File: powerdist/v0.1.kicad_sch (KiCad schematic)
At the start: 29 parts, among them J1 Conn_01x02_Socket, J2 Conn_01x02_Socket, J3 Conn_01x02_Socket, J4 Conn_01x02_Socket

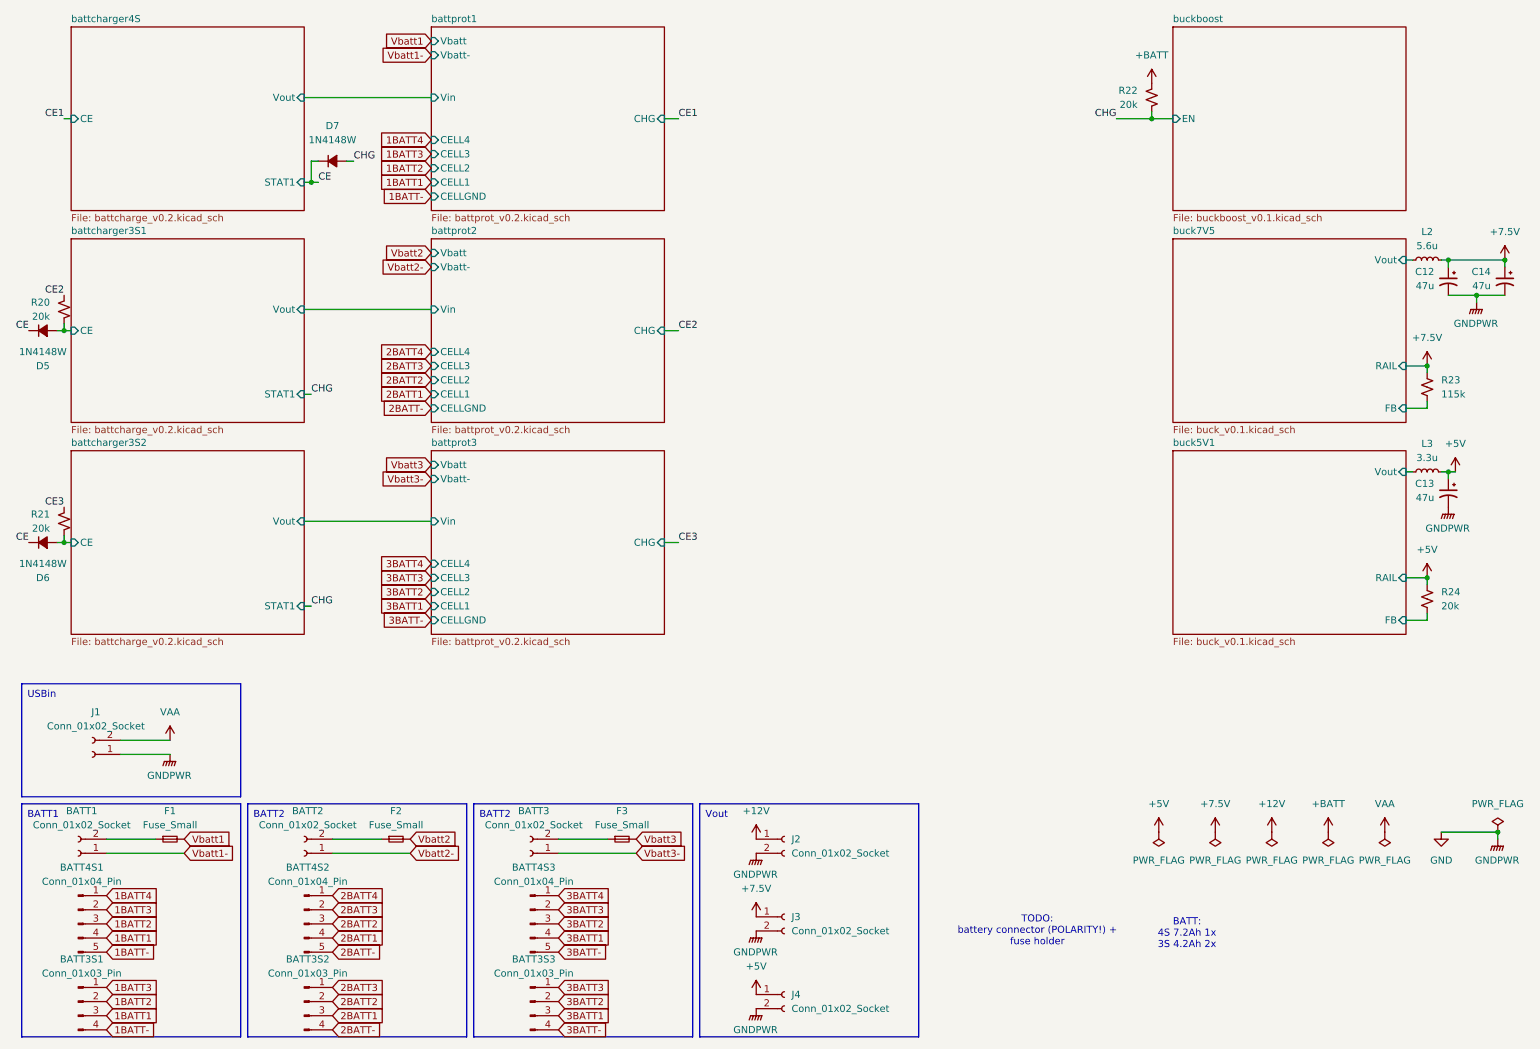
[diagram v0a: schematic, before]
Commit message: local 19/10
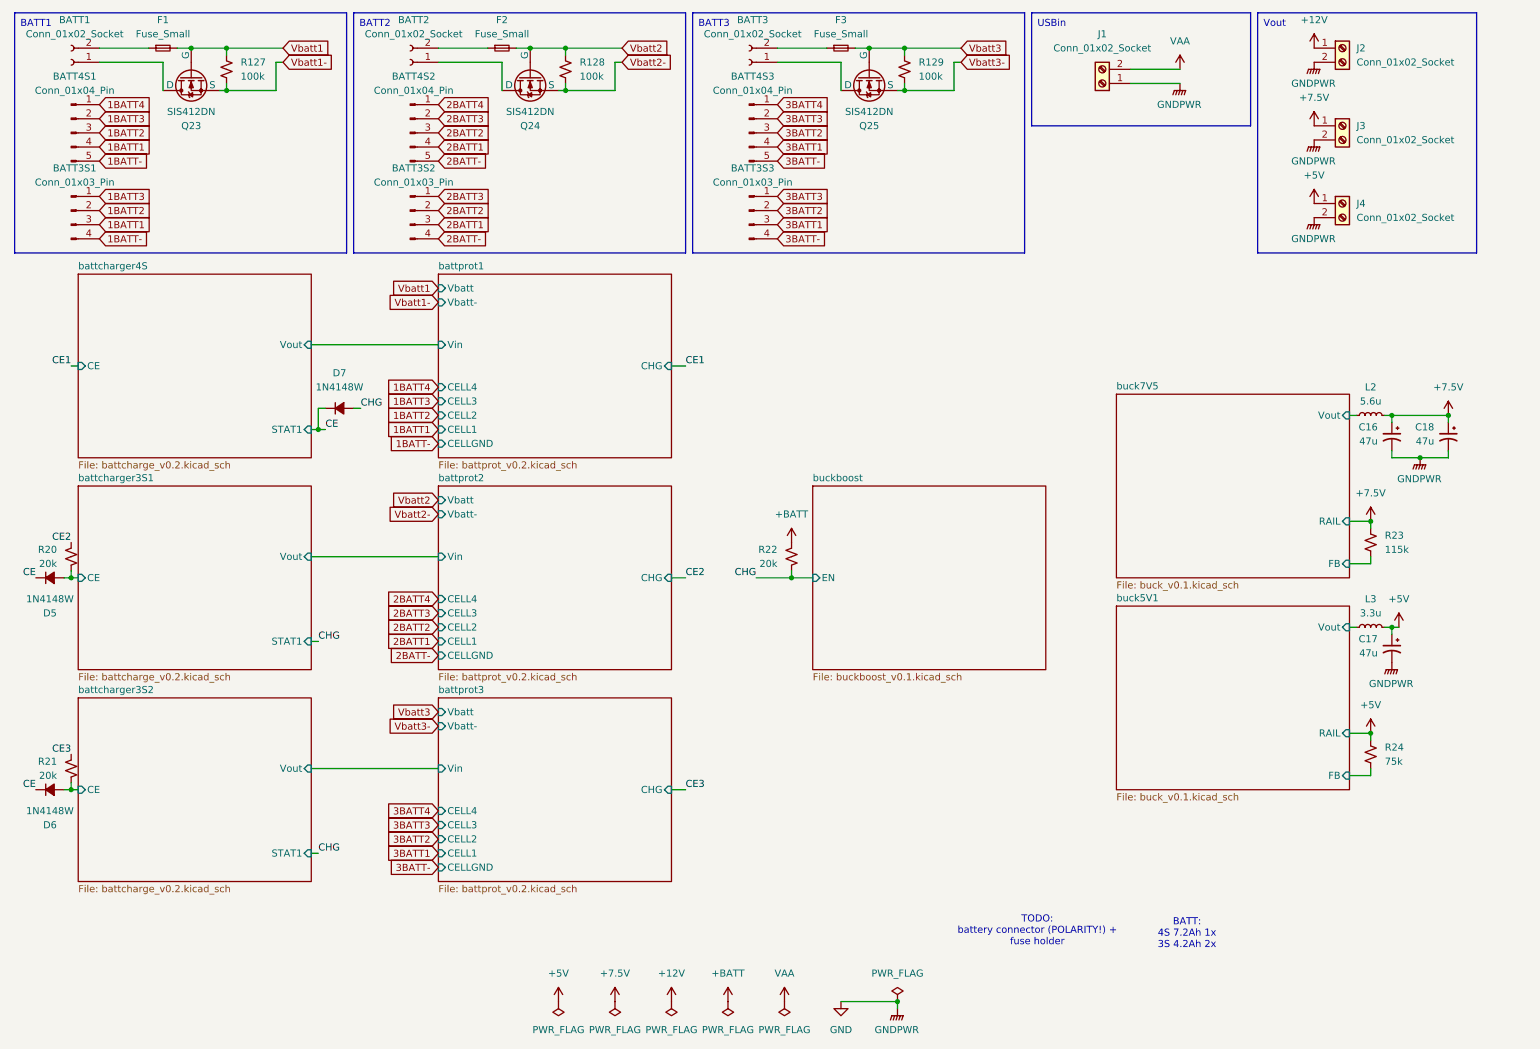
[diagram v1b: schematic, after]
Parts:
- added Q23, Q24, Q25: SIS412DN, symbol Simulation_SPICE:NMOS
- added R127, R128, R129: 100k, symbol Device:R_Small_US
- BATT1, BATT2, BATT3: footprint (none) -> Connector:Banana_Jack_2Pin
- BATT3S1, BATT3S2, BATT3S3: footprint (none) -> Connector_JST:JST_XH_B4B-XH-AM_1x04_P2.50mm_Vertical
- BATT4S1, BATT4S2, BATT4S3: footprint (none) -> Connector_JST:JST_XH_B5B-XH-AM_1x05_P2.50mm_Vertical
- J1, J2, J3, J4: symbol Connector:Conn_01x02_Socket -> Connector:Screw_Terminal_01x02
- R24: value 20k -> 75k
- renumbered C12 to C16, C13 to C17, C14 to C18
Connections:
- net Vbatt1: now also Q23.2 (G), R127.1
- net Vbatt1-: now also Q23.3 (S), R127.2; no longer BATT1.1 (Pin_1)
- net Vbatt2: now also Q24.2 (G), R128.1
- net Vbatt2-: now also Q24.3 (S), R128.2; no longer BATT2.1 (Pin_1)
- net Vbatt3: now also Q25.2 (G), R129.1
- net Vbatt3-: now also Q25.3 (S), R129.2; no longer BATT3.1 (Pin_1)
- new net: BATT1.1 (Pin_1), Q23.1 (D)
- new net: BATT2.1 (Pin_1), Q24.1 (D)
- new net: BATT3.1 (Pin_1), Q25.1 (D)
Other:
- moved on the sheet: BATT1, BATT2, BATT3, BATT3S1, BATT3S2, BATT3S3, BATT4S1, BATT4S2, BATT4S3, C16, C17, C18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

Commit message: lab 20/10
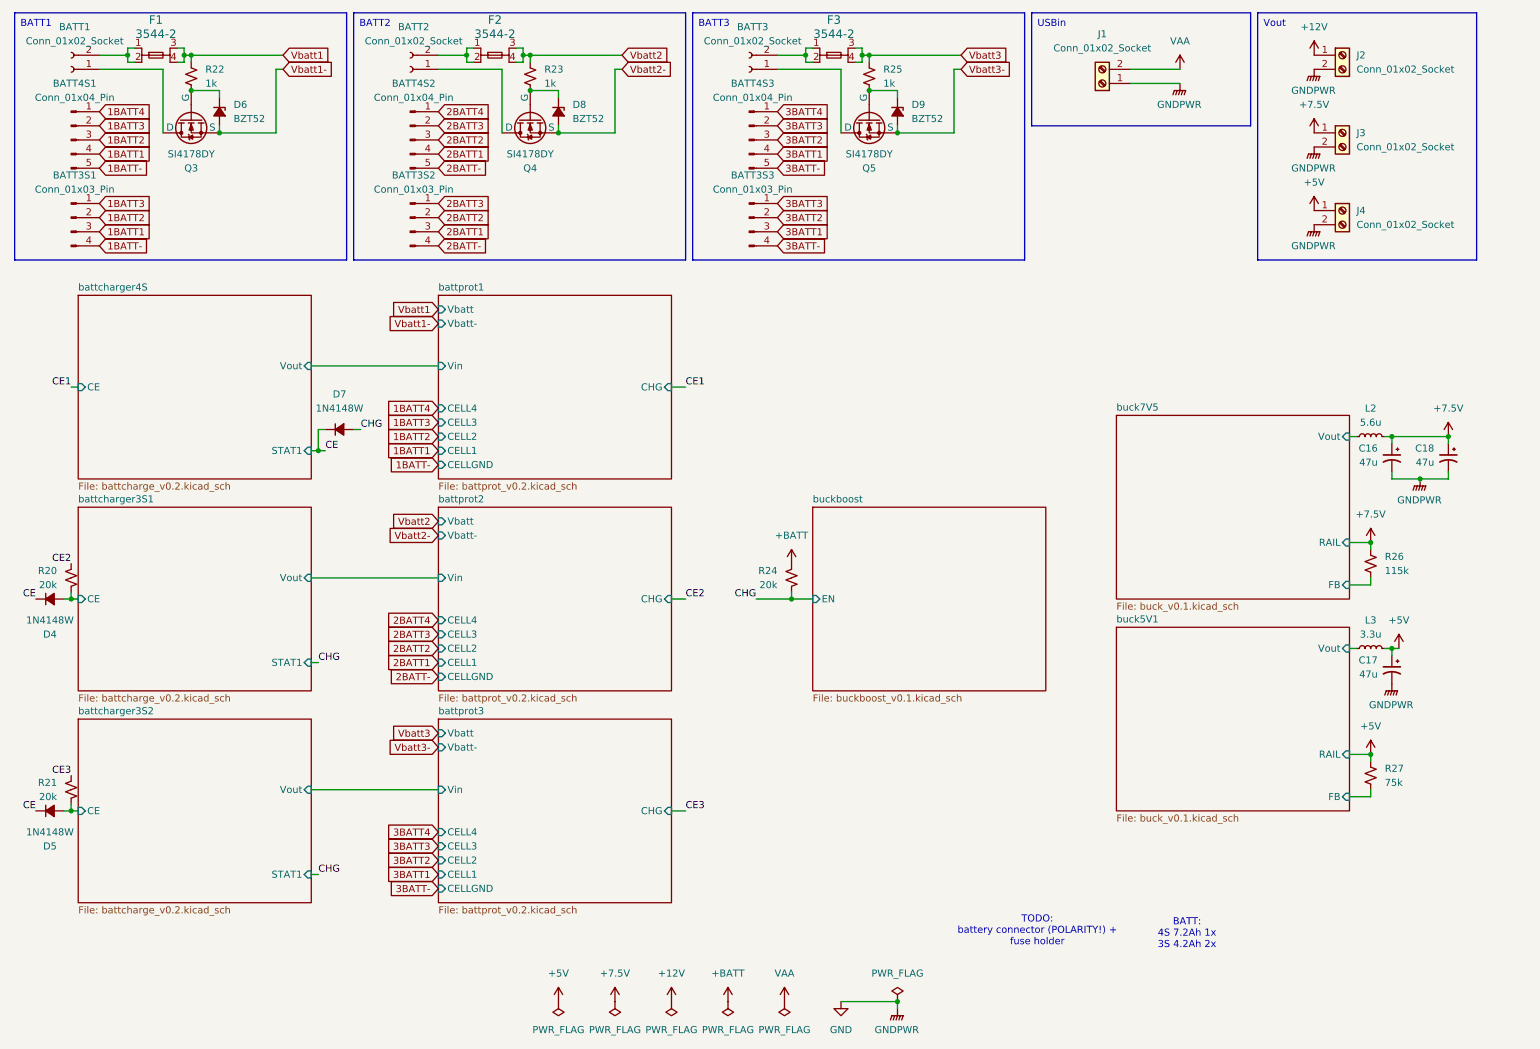
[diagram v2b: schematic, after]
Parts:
- removed F1, F2, F3: Fuse_Small, symbol Device:Fuse_Small
- removed Q24, Q25: SIS412DN, symbol Simulation_SPICE:NMOS
- removed R127, R128, R129: 100k, symbol Device:R_Small_US
- added D6, D8, D9: BZT52, symbol Device:D_Zener_Small_Filled
- added F1, F2, F3: 3544-2, powerdist:CONN_3544-2_KEY, symbol 3544-2:3544-2
- added Q4, Q5: SI4178DY, symbol Simulation_SPICE:NMOS
- added R22, R23, R25: 1k, symbol Device:R_Small_US
- Q3: renamed from Q23; value SIS412DN -> SI4178DY
- renumbered D5 to D4, D6 to D5, R22 to R24, R23 to R26, R24 to R27
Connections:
- net Vbatt1: now also F1.3, F1.4, R22.1; no longer Q3.2 (G)
- net Vbatt1-: now also D6.2 (A)
- net Vbatt2: now also F2.3, F2.4, R23.1
- net Vbatt2-: now also D8.2 (A), Q4.3 (S)
- net Vbatt3: now also F3.3, F3.4, R25.1
- net Vbatt3-: now also D9.2 (A), Q5.3 (S)
- net at BATT1.2 (Pin_2): now also F1.1, F1.2
- net at BATT3.2 (Pin_2): now also F3.1, F3.2
- net at BATT2.1 (Pin_1): now also Q4.1 (D)
- net at BATT2.2 (Pin_2): now also F2.1, F2.2
- net at BATT3.1 (Pin_1): now also Q5.1 (D)
- new net: D8.1 (K), Q4.2 (G), R23.2
- new net: D9.1 (K), Q5.2 (G), R25.2
- new net: D6.1 (K), Q3.2 (G), R22.2
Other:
- moved on the sheet: BATT1, BATT2, BATT3, BATT3S1, BATT3S2, BATT3S3, BATT4S1, BATT4S2, BATT4S3, C16, C17, C18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
